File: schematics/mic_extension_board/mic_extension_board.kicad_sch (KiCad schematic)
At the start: 22 parts, among them J2 Conn_01x02_Male, J9 Conn_01x03_Female, U10 LM4881M/NOPB, U3 k7833, U7 MC78M09_TO252, U8 MC78M05_TO252

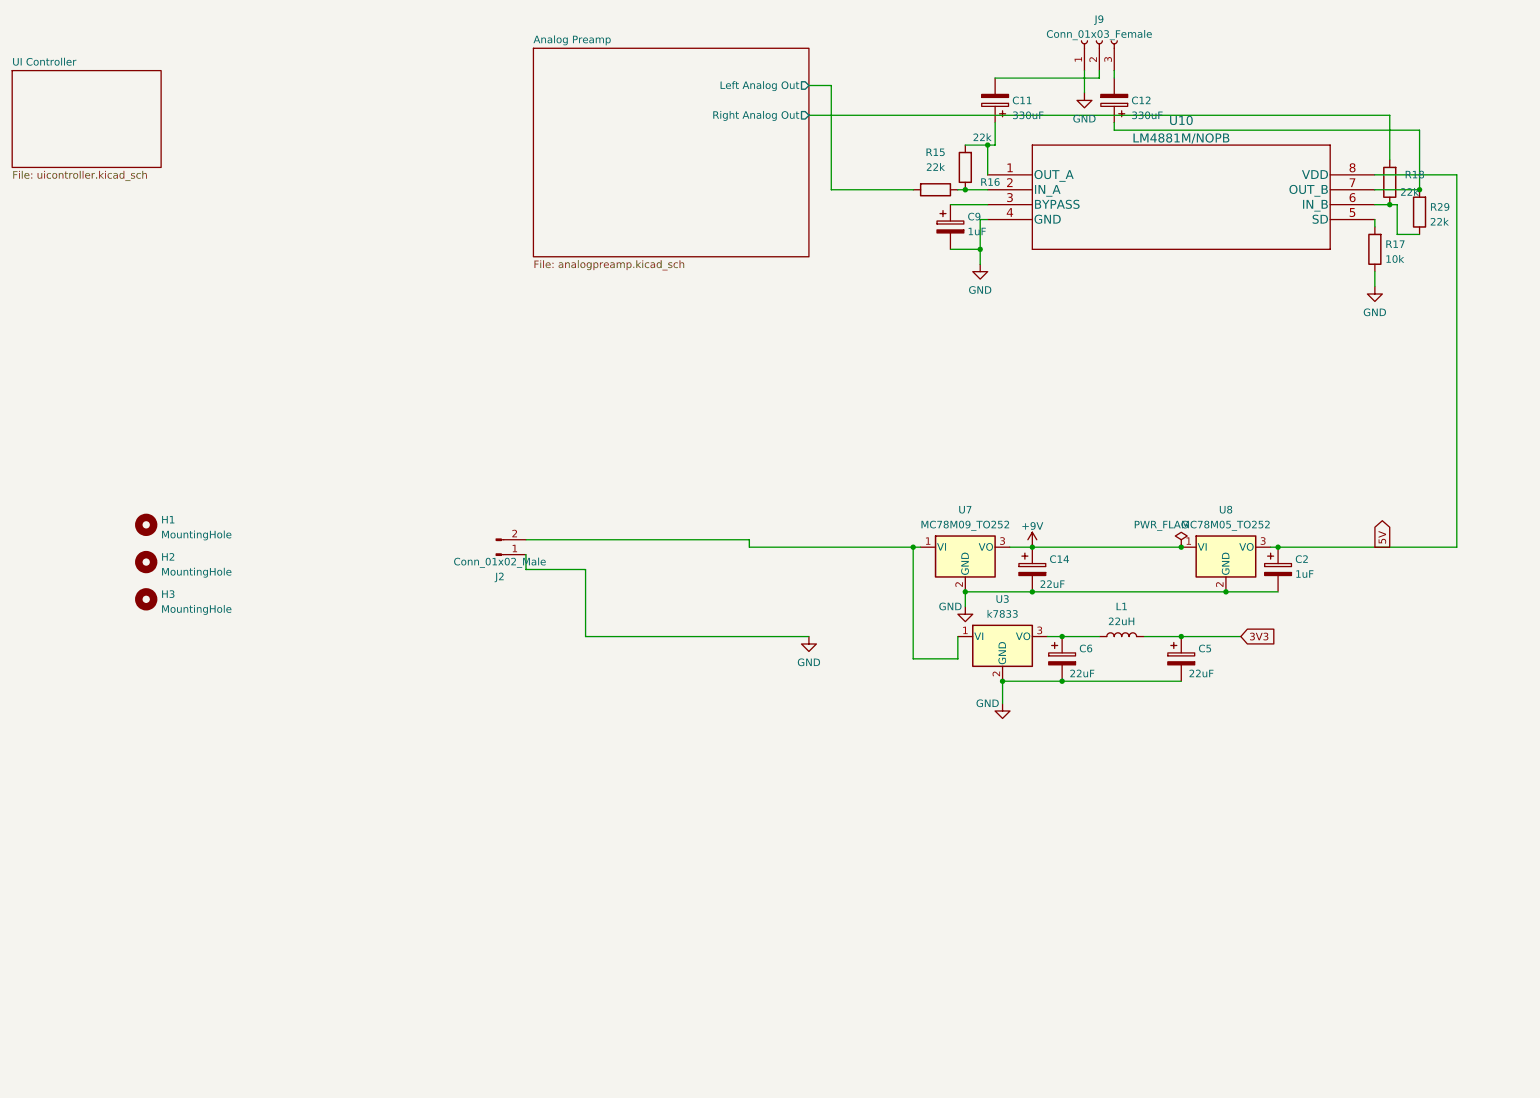
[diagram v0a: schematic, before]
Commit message: more layouting
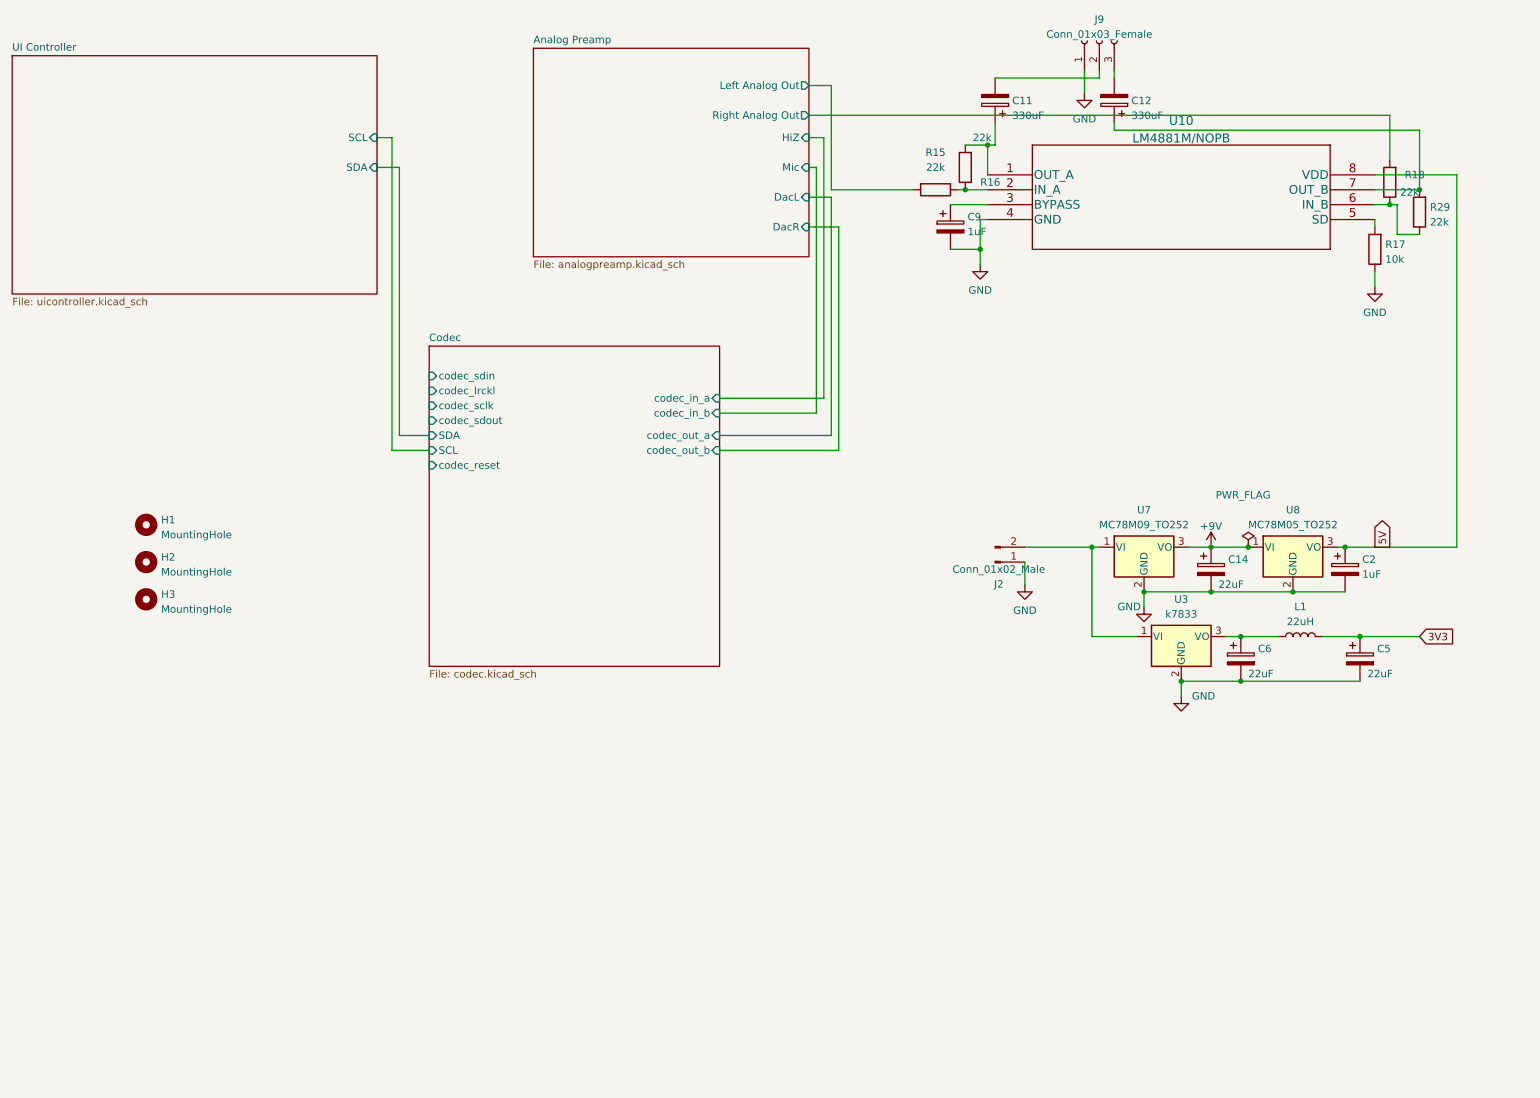
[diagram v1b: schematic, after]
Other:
- added sheet Codec (codec.kicad_sch)
- sheet Analog Preamp ports: added DacL, DacR, HiZ, Mic; removed none
- sheet UI Controller ports: added SCL, SDA; removed none
- moved on the sheet: C14, C2, C5, C6, J2, L1, U3, U7, U8

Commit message: finished full board
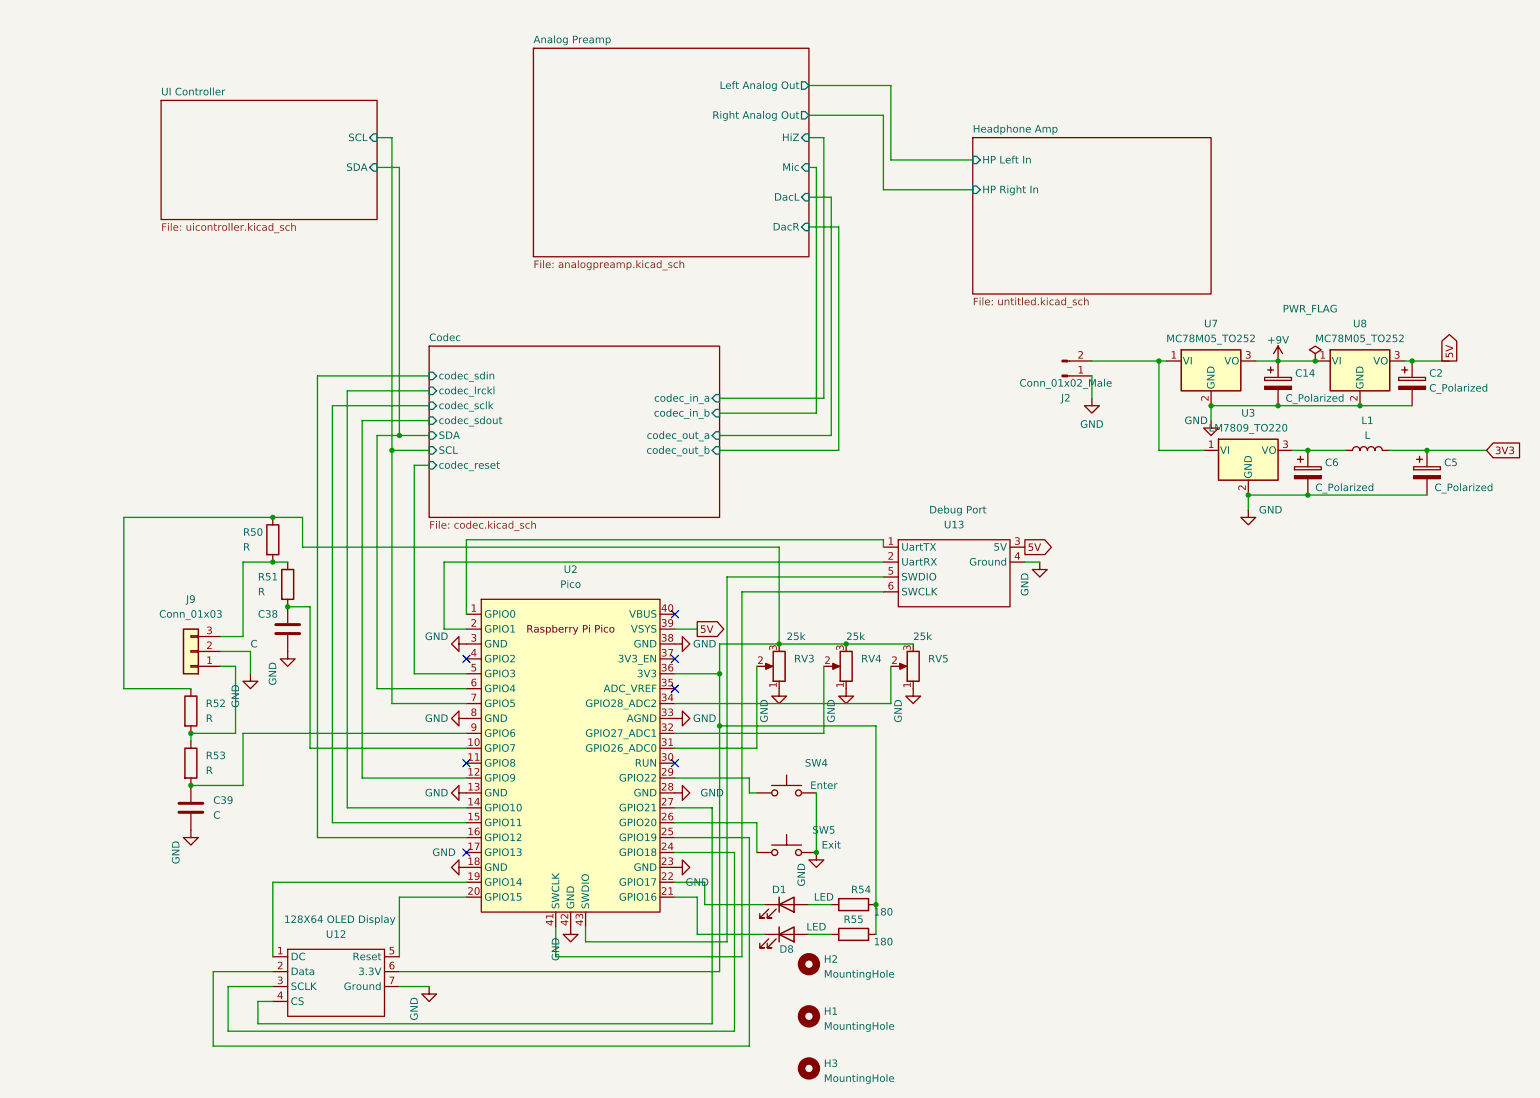
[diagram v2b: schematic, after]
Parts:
- removed C11, C12: 330uF, Capacitor_SMD:CP_Elec_6.3x7.7, symbol Device:C_Polarized
- removed C9: 1uF, Capacitor_SMD:CP_Elec_4x4.5, symbol Device:C_Polarized
- removed J9: Conn_01x03_Female, Connector_PinHeader_2.54mm:PinHeader_1x03_P2.54mm_Vertical, symbol Connector:Conn_01x03_Female
- removed R15, R16, R18, R29: 22k, Resistor_SMD:R_0603_1608Metric_Pad0.98x0.95mm_HandSolder, symbol Device:R
- removed R17: 10k, Resistor_SMD:R_0603_1608Metric_Pad0.98x0.95mm_HandSolder, symbol Device:R
- removed U10: LM4881M/NOPB, Package_SO:SOIC-8_3.9x4.9mm_P1.27mm, symbol 2023-02-24_23-31-36:LM4881M/NOPB
- added C38, C39: C, Capacitor_SMD:C_0805_2012Metric_Pad1.18x1.45mm_HandSolder, symbol Device:C
- added D1, D8: LED, Connector_PinHeader_2.54mm:PinHeader_1x02_P2.54mm_Vertical, symbol Device:LED
- added J9: Conn_01x03, Connector_PinHeader_2.54mm:PinHeader_1x03_P2.54mm_Vertical, symbol Connector_Generic:Conn_01x03
- added R50, R51, R52, R53: R, Resistor_SMD:R_0603_1608Metric_Pad0.98x0.95mm_HandSolder, symbol Device:R
- added R54, R55: 180, Resistor_SMD:R_0603_1608Metric_Pad0.98x0.95mm_HandSolder, symbol Device:R
- added RV3, RV4, RV5: 25k, Connector_PinHeader_2.54mm:PinHeader_1x03_P2.54mm_Vertical, symbol Device:R_Potentiometer
- added SW4: Enter, Connector_PinHeader_2.54mm:PinHeader_1x02_P2.54mm_Vertical, symbol Switch:SW_Push
- added SW5: Exit, Connector_PinHeader_2.54mm:PinHeader_1x02_P2.54mm_Vertical, symbol Switch:SW_Push
- added U12: 128X64 OLED Display, Connector_PinHeader_2.54mm:PinHeader_1x07_P2.54mm_Vertical, symbol GraphicDisplay:128X64_OLED_Display
- added U13: Debug Port, Connector_PinHeader_2.54mm:PinHeader_1x06_P2.54mm_Vertical, symbol GraphicDisplay:DebugPort
- added U2: Pico, MCU_RaspberryPi_and_Boards:RPi_Pico_SMD_TH, symbol Raspberry Pi Pico:Pico
- C14, C5, C6: value 22uF -> C_Polarized
- C2: value 1uF -> C_Polarized
- L1: value 22uH -> L
- U3: value k7833 -> LM7809_TO220; footprint Connector_PinHeader_2.54mm:PinHeader_1x03_P2.54mm_Vertical -> Package_TO_SOT_THT:TO-220-3_Vertical
- U7: value MC78M09_TO252 -> MC78M05_TO252
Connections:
- net 5V: now also U13.3 (5V), U2.39 (VSYS)
- net Codec/SCL: now also U2.7 (GPIO5)
- net Codec/SDA: now also U2.6 (GPIO4)
- net Codec/codec_lrckl: now also U2.14 (GPIO10)
- net Codec/codec_reset: now also U2.5 (GPIO3)
- net Codec/codec_sclk: now also U2.15 (GPIO11)
- net Codec/codec_sdin: now also U2.16 (GPIO12)
- net Codec/codec_sdout: now also U2.12 (GPIO9)
- net GND: now also C38.2, C39.2, J9.2 (Pin_2), RV3.1, RV4.1, RV5.1, SW4.2, SW5.2, U12.7 (Ground), U13.4 (Ground), U2.13 (GND), U2.18 (GND), U2.23 (GND), U2.28 (GND), U2.3 (GND), U2.33 (AGND), U2.38 (GND), U2.42 (GND), U2.8 (GND)
- new net: U13.1 (UartTX), U2.1 (GPIO0)
- new net: C38.1, R51.2, U2.10 (GPIO7)
- new net: U12.1 (DC), U2.19 (GPIO14)
- new net: U13.2 (UartRX), U2.2 (GPIO1)
- new net: U12.5 (Reset), U2.20 (GPIO15)
- new net: D8.1 (K), U2.21 (GPIO16)
- new net: D1.1 (K), U2.22 (GPIO17)
- new net: U12.3 (SCLK), U2.24 (GPIO18)
- new net: U12.2 (Data), U2.25 (GPIO19)
- new net: SW5.1, U2.26 (GPIO20)
- new net: U12.4 (CS), U2.27 (GPIO21)
- new net: SW4.1, U2.29 (GPIO22)
- new net: RV3.2, U2.31 (GPIO26_ADC0)
- new net: RV4.2, U2.32 (GPIO27_ADC1)
- new net: RV5.2, U2.34 (GPIO28_ADC2)
- new net: R50.1, R52.1, R54.2, R55.2, RV3.3, RV4.3, RV5.3, U12.6 (3.3V), U2.36 (3V3)
- new net: U13.6 (SWCLK), U2.41 (SWCLK)
- new net: U13.5 (SWDIO), U2.43 (SWDIO)
- new net: C39.1, R53.2, U2.9 (GPIO6)
- new net: J9.3 (Pin_3), R50.2, R51.1
- new net: D8.2 (A), R55.1
- new net: J9.1 (Pin_1), R52.2, R53.1
- new net: D1.2 (A), R54.1
- no-connect marks 0 -> 7
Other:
- added sheet Headphone Amp (untitled.kicad_sch)
- moved on the sheet: C14, C2, C5, C6, H1, H2, H3, J2, L1, U3, U7, U8
